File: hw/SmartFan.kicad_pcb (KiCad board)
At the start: 2 copper layers, 115 x 56 mm, 60 parts, among them J1 Barrel_Jack, J2 JTAG_SWD, J3 BTLE_LED_Conn, J4 ANT_LED_Conn, J5 RGB_LED_Conn, J6 PB_Conn, J7 FAN_CONN, Q1 MMBT2222A-7-F, Q2 MMBT2222A-7-F, Q3 MMBT2222A-TP, Q4 MMBT2222A-TP, Q5 MMBT2222A-TP, Q6 MMBT2222A-7-F, Q7 MMBT2222A-7-F, Q8 MMBT2222A-7-F, U1 L7805CV, U2 LTV-816S-TA1, U3 LTV-816S-TA1, U4 LTV-816S-TA1, U5 LD1117S33CTR

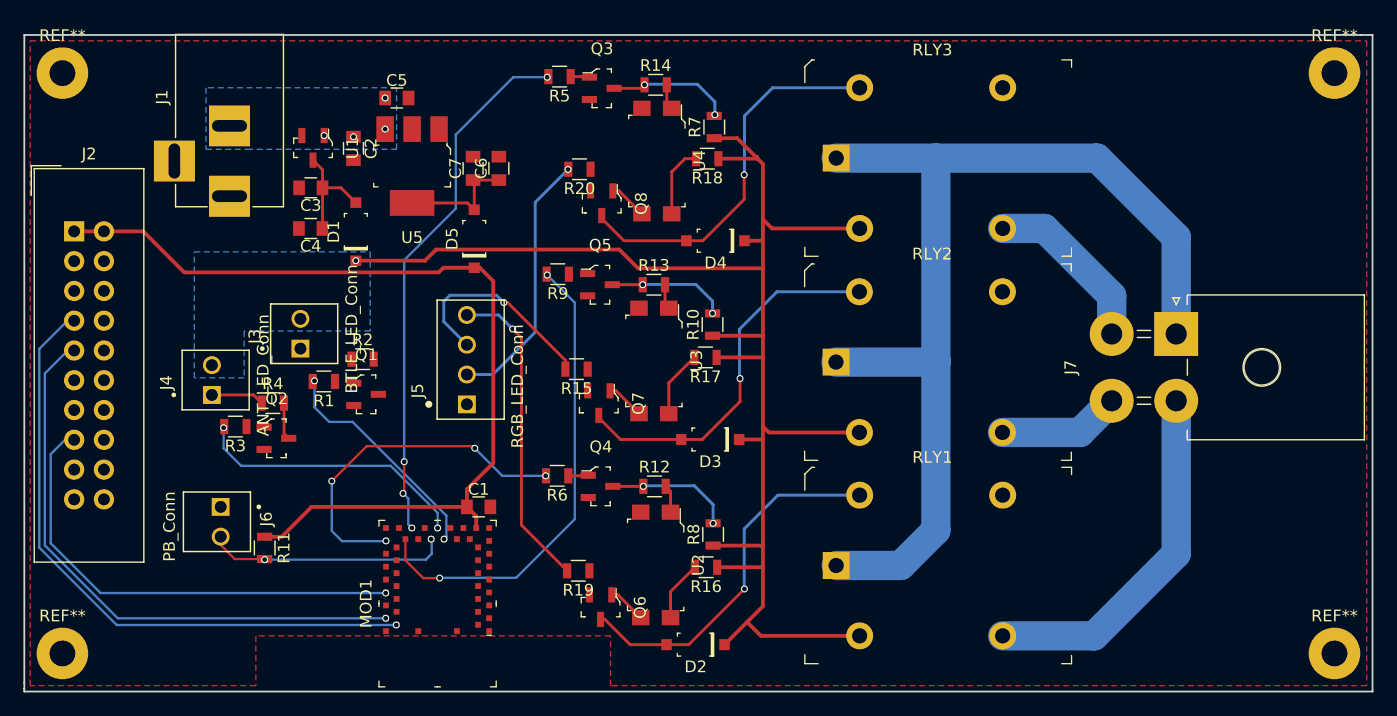
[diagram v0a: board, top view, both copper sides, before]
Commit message: Updates to PCB layout
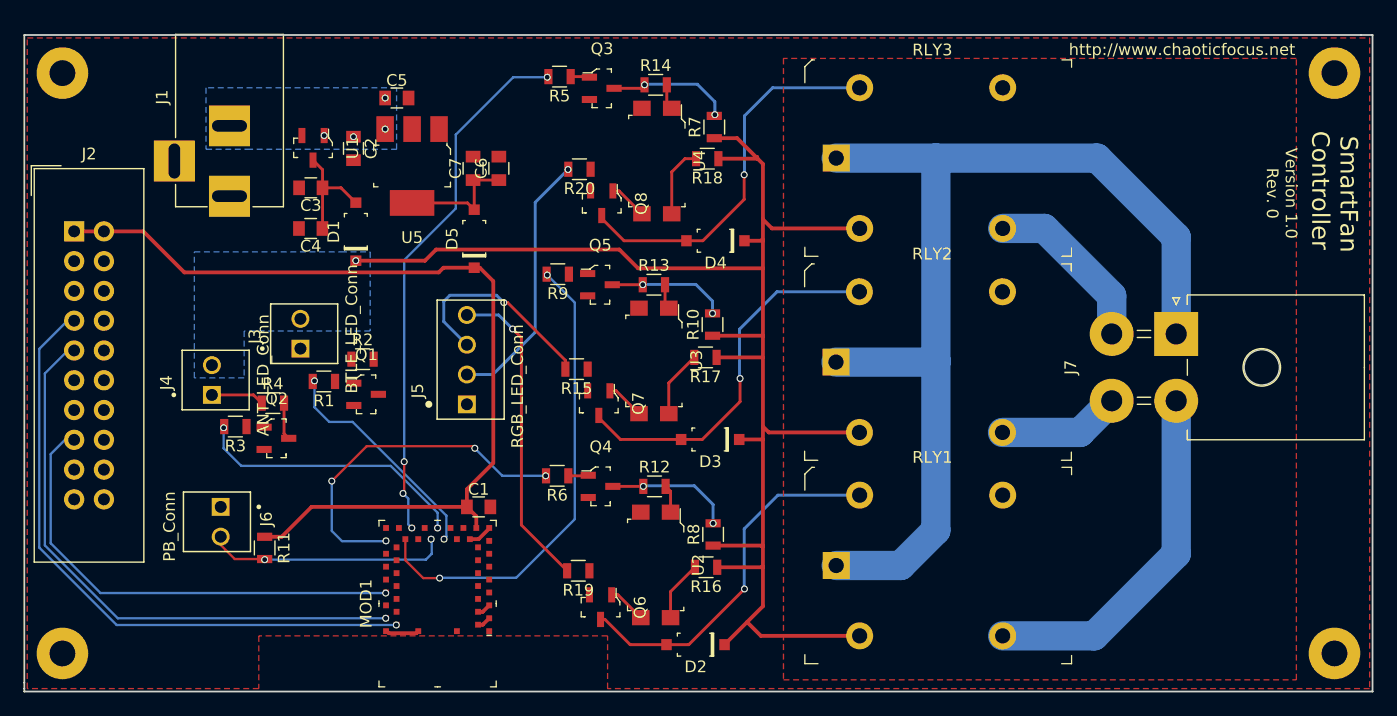
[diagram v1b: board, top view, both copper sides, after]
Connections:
- REF** pad 1: (no net) -> GND (x4)
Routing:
- net GND: track 0.00 -> 7.32 mm
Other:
- board text added: "SmartFan Controller"
- board text added: "Version 1.0 Rev. 0"
- board text added: "http://www.chaoticfocus.net"
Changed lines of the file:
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@@
 (kicad_pcb (version 4) (host pcbnew 4.0.7-e2-6376~61~ubuntu18.04.1)
   (general
-    (links 124)
-    (no_connects 8)
+    (links 128)
+    (no_connects 5)
     (area 111.924999 79.924999 227.075001 136.075001)
     (thickness 1.6)
-    (drawings 7)
-    (tracks 302)
+    (drawings 10)
+    (tracks 313)
     (zones 0)
     (modules 60)
@@
     (tags "mounting hole 2.2mm m2")
     (attr virtual)
-    (fp_text reference REF** (at 0 -3.2) (layer F.SilkS)
+    (fp_text reference REF** (at 0 -3.2) (layer F.SilkS) hide
       (effects (font (size 1 1) (thickness 0.15)))
     )
@@
     (fp_circle (center 0 0) (end 2.2 0) (layer Cmts.User) (width 0.15))
     (fp_circle (center 0 0) (end 2.45 0) (layer F.CrtYd) (width 0.05))
-    (pad 1 thru_hole circle (at 0 0) (size 4.4 4.4) (drill 2.2) (layers *.Cu *.Mask))
+    (pad 1 thru_hole circle (at 0 0) (size 4.4 4.4) (drill 2.2) (layers *.Cu *.Mask)
+      (net 2 GND))
   )
   (module Mounting_Holes:MountingHole_2.2mm_M2_Pad (layer F.Cu)
@@
     (tags "mounting hole 2.2mm m2")
     (attr virtual)
-    (fp_text reference REF** (at 0 -3.2) (layer F.SilkS)
+    (fp_text reference REF** (at 0 -3.2) (layer F.SilkS) hide
       (effects (font (size 1 1) (thickness 0.15)))
     )
@@
       (effects (font (size 1 1) (thickness 0.15)))
     )
-    (fp_text user %R (at 0.3 0) (layer F.Fab)
+    (fp_text user %R (at 0.3 0) (layer F.Fab) hide
       (effects (font (size 1 1) (thickness 0.15)))
     )
     (fp_circle (center 0 0) (end 2.2 0) (layer Cmts.User) (width 0.15))
     (fp_circle (center 0 0) (end 2.45 0) (layer F.CrtYd) (width 0.05))
-    (pad 1 thru_hole circle (at 0 0) (size 4.4 4.4) (drill 2.2) (layers *.Cu *.Mask))
+    (pad 1 thru_hole circle (at 0 0) (size 4.4 4.4) (drill 2.2) (layers *.Cu *.Mask)
+      (net 2 GND))
   )
   (module Mounting_Holes:MountingHole_2.2mm_M2_Pad (layer F.Cu)
@@
     (tags "mounting hole 2.2mm m2")
     (attr virtual)
-    (fp_text reference REF** (at 0 -3.2) (layer F.SilkS)
+    (fp_text reference REF** (at 0 -3.2) (layer F.SilkS) hide
       (effects (font (size 1 1) (thickness 0.15)))
     )
@@
     (fp_circle (center 0 0) (end 2.2 0) (layer Cmts.User) (width 0.15))
     (fp_circle (center 0 0) (end 2.45 0) (layer F.CrtYd) (width 0.05))
-    (pad 1 thru_hole circle (at 0 0) (size 4.4 4.4) (drill 2.2) (layers *.Cu *.Mask))
+    (pad 1 thru_hole circle (at 0 0) (size 4.4 4.4) (drill 2.2) (layers *.Cu *.Mask)
+      (net 2 GND))
   )
   (module Mounting_Holes:MountingHole_2.2mm_M2_Pad (layer F.Cu)
@@
     (tags "mounting hole 2.2mm m2")
     (attr virtual)
-    (fp_text reference REF** (at 0 -3.2) (layer F.SilkS)
+    (fp_text reference REF** (at 0 -3.2) (layer F.SilkS) hide
       (effects (font (size 1 1) (thickness 0.15)))
     )
@@
       (effects (font (size 1 1) (thickness 0.15)))
     )
-    (fp_text user %R (at 0.3 0) (layer F.Fab)
+    (fp_text user %R (at 0.3 0) (layer F.Fab) hide
       (effects (font (size 1 1) (thickness 0.15)))
     )
     (fp_circle (center 0 0) (end 2.2 0) (layer Cmts.User) (width 0.15))
     (fp_circle (center 0 0) (end 2.45 0) (layer F.CrtYd) (width 0.05))
-    (pad 1 thru_hole circle (at 0 0) (size 4.4 4.4) (drill 2.2) (layers *.Cu *.Mask))
+    (pad 1 thru_hole circle (at 0 0) (size 4.4 4.4) (drill 2.2) (layers *.Cu *.Mask)
+      (net 2 GND))
+  )
+  (gr_text http://www.chaoticfocus.net (at 210.75 81.25) (layer F.SilkS)
+    (effects (font (size 1 1) (thickness 0.25)))
+  )
+  (gr_text "Version 1.0\nRev. 0" (at 219.25 93.5 270) (layer F.SilkS)
+    (effects (font (size 1 1) (thickness 0.25)))
+  )
+  (gr_text " SmartFan \nController" (at 223.75 93.25 270) (layer F.SilkS)
+    (effects (font (size 1.5 1.5) (thickness 0.3)))
   )
   (gr_line (start 112 80) (end 226 80) (angle 90) (layer Edge.Cuts) (width 0.15))
@@
   (segment (start 152 116.5) (end 149.75 118.75) (width 0.325) (layer F.Cu) (net 1))
   (segment (start 149.75 118.75) (end 149.75 120.25) (width 0.325) (layer F.Cu) (net 1))
+  (segment (start 142.85 130.85) (end 142.925 130.85) (width 0.325) (layer F.Cu) (net 2))
+  (segment (start 142.925 130.85) (end 143.1 131.025) (width 0.325) (layer F.Cu) (net 2))
+  (segment (start 143.1 131.025) (end 145.425 131.025) (width 0.325) (layer F.Cu) (net 2))
+  (segment (start 145.425 131.025) (end 145.6 130.85) (width 0.325) (layer F.Cu) (net 2))
+  (segment (start 151.65 122.05) (end 151.65 122.1) (width 0.325) (layer F.Cu) (net 2))
+  (segment (start 151.65 122.1) (end 150.75 123) (width 0.325) (layer F.Cu) (net 2))
+  (segment (start 150.75 123) (end 150 123) (width 0.325) (layer F.Cu) (net 2))
+  (segment (start 150.7 130.3) (end 151.1 130.3) (width 0.325) (layer F.Cu) (net 2))
+  (segment (start 151.1 130.3) (end 151.65 129.75) (width 0.325) (layer F.Cu) (net 2))
+  (segment (start 150.7 129.2) (end 151.1 129.2) (width 0.325) (layer F.Cu) (net 2))
+  (segment (start 151.1 129.2) (end 151.65 128.65) (width 0.325) (layer F.Cu) (net 2))
   (segment (start 140.275 99.25) (end 146.175 99.25) (width 0.325) (layer F.Cu) (net 3))
   (segment (start 164.35 99.9) (end 175 99.9) (width 0.325) (layer F.Cu) (net 3))
@@
     )
   )
-  (zone (net 2) (net_name GND) (layer F.Cu) (hatch edge 0.508)
-    (connect_pads (clearance 0.508))
-    (min_thickness 0.254)
-    (fill yes (arc_segments 16) (thermal_gap 0.508) (thermal_bridge_width 0.508))
-    (polygon
-      (pts
-        (xy 226.5 135.5) (xy 162 135.5) (xy 162 131.25) (xy 131.75 131.25) (xy 131.75 135.5)
-        (xy 112.5 135.5) (xy 112.5 80.5) (xy 226.5 80.5)
-      )
-    )
-  )
   (zone (net 64) (net_name +9V) (layer B.Cu) (hatch edge 0.508)
     (connect_pads (clearance 0.508))
@@
       )
     )
+  )
+  (zone (net 2) (net_name GND) (layer F.Cu) (hatch edge 0.508)
+    (connect_pads (clearance 0.508))
+    (min_thickness 0.254)
+    (fill yes (arc_segments 16) (thermal_gap 0.508) (thermal_bridge_width 0.508))
+    (polygon
+      (pts
+        (xy 226.75 80.25) (xy 226.75 135.75) (xy 161.75 135.75) (xy 161.75 131.25) (xy 132 131.25)
+        (xy 132 135.75) (xy 112.25 135.75) (xy 112.25 80.25) (xy 176.75 80.25)
+      )
+    )
+    (polygon
+      (pts        (xy 220.5 135) (xy 220.5 82) (xy 176.75 82) (xy 176.75 135)
+      )
+    )
